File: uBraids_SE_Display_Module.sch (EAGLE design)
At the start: 32 parts, among them Q1 NPN-SOT323-BEC, Q2 NPN-SOT323-BEC, Q3 NPN-SOT323-BEC, Q4 NPN-SOT323-BEC, U1 SN74HC595-TSSOP-16, U2 SN74HC595-TSSOP-16

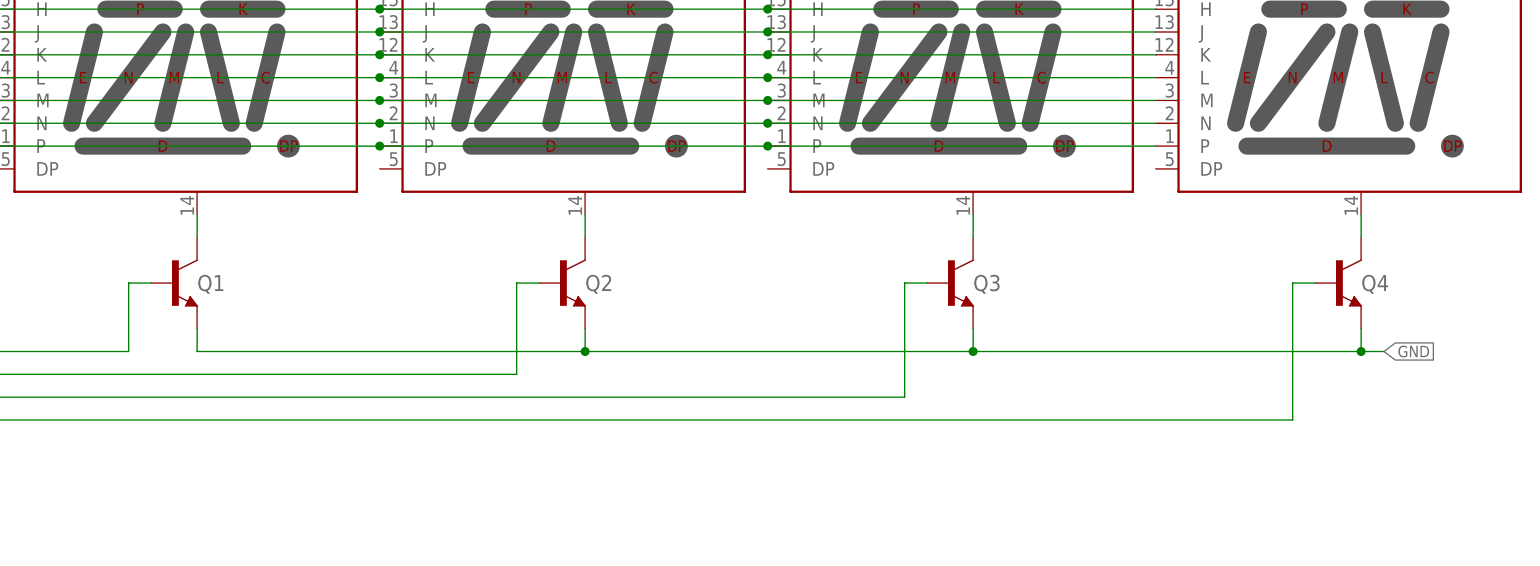
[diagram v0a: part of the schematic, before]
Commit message: prep for production of revision C
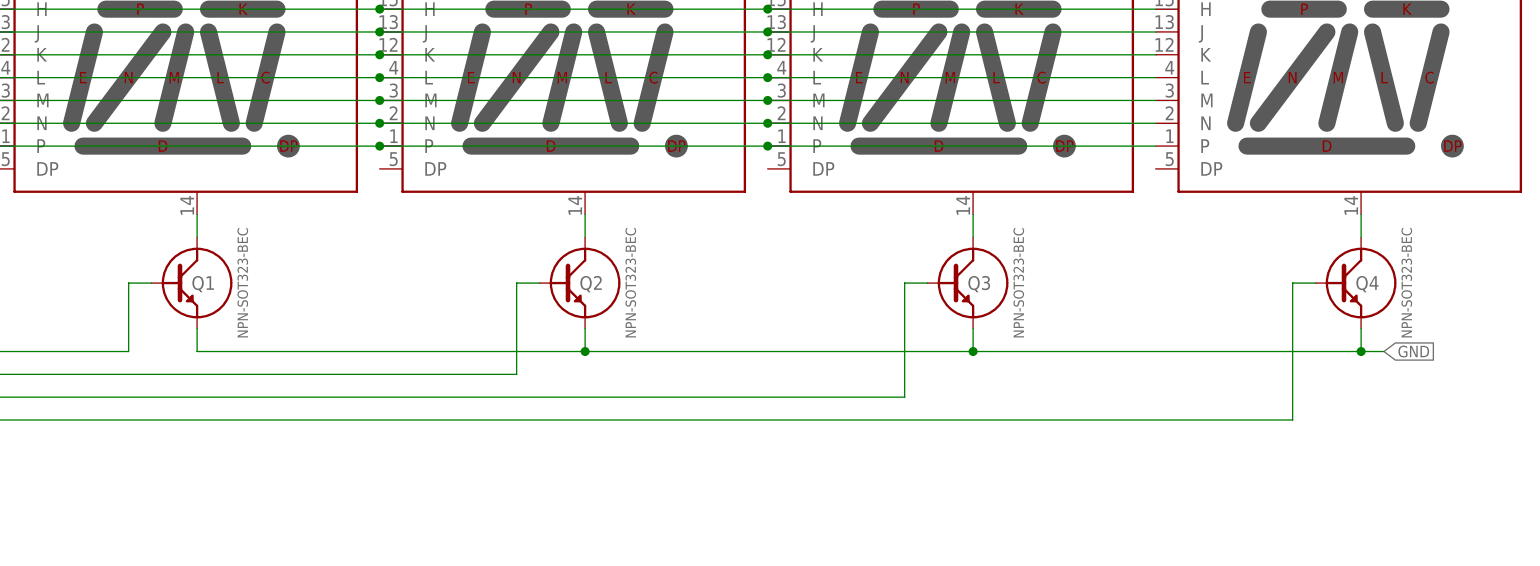
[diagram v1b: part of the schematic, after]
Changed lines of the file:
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@@
 with this version.
+</note>
+<note version="8.3" severity="warning">
+Since Version 8.3, EAGLE supports URNs for individual library
+assets (packages, symbols, and devices). The URNs of those assets
+will not be understood (or retained) with this version.
 </note>
 </compatibility>
